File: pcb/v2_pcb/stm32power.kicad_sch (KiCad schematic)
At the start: 64 parts, among them U1 STM32N657X0H3Q

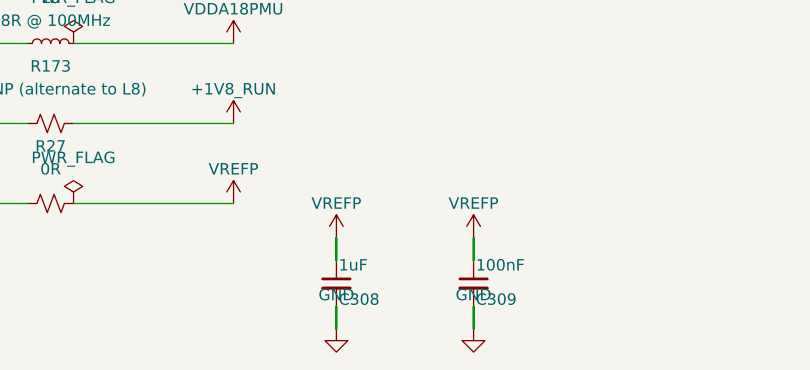
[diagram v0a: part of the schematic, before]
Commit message: power and debug cleanup
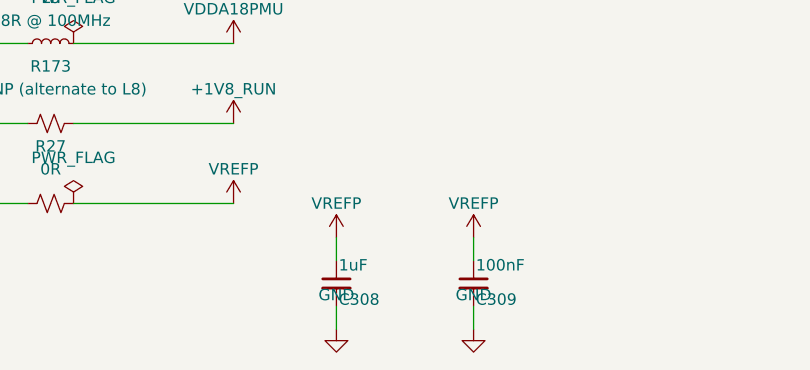
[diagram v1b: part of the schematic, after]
